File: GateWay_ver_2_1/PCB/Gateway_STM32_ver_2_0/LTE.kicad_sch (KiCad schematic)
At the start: 37 parts, among them J3 SIM_Card, Q2 MMBT3904, Q3 AO3400, Q4 AO3400, U6 SIM7600E-H

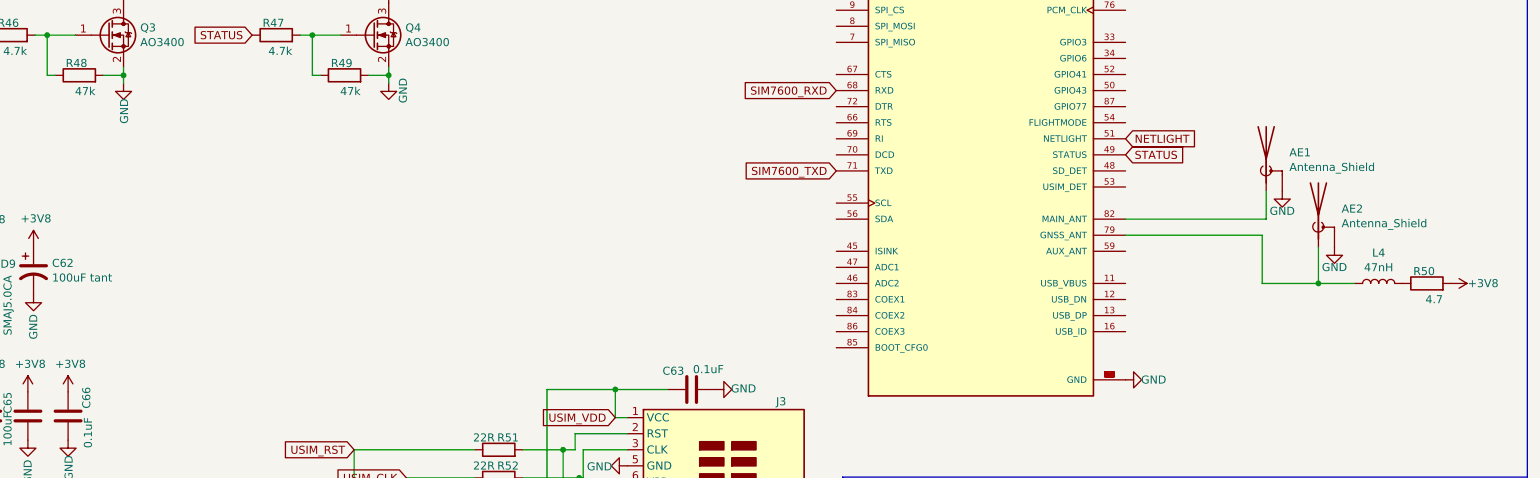
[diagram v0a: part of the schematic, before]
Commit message: 1
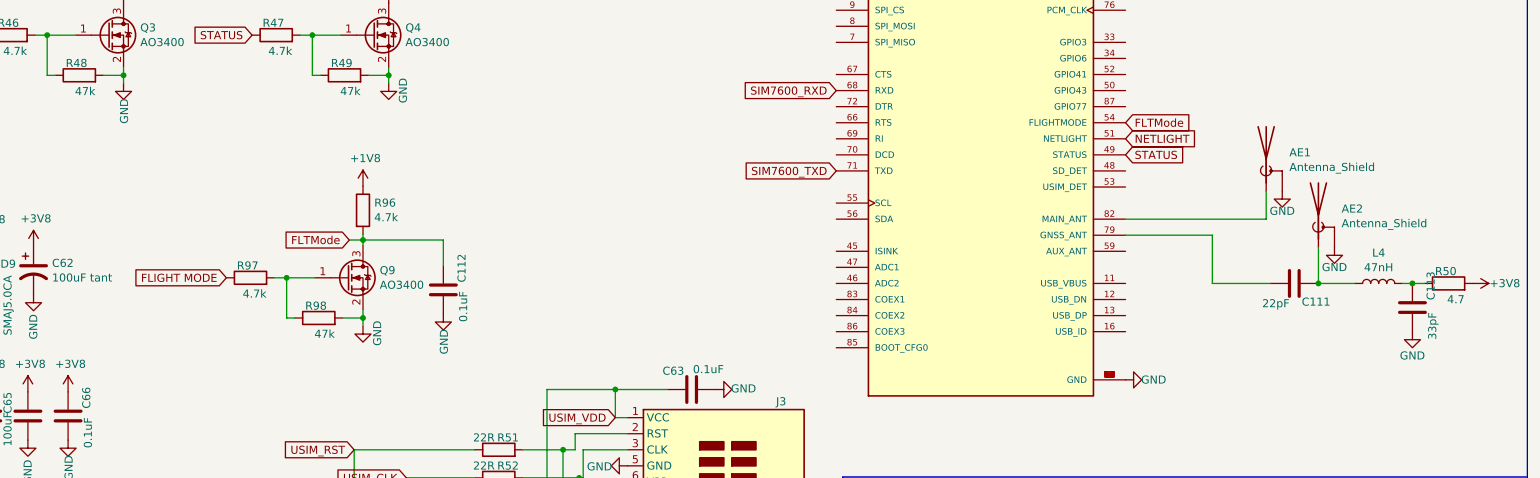
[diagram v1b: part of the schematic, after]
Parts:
- added C111: 22pF, Capacitor_SMD:C_0603_1608Metric, symbol Device:C
- added C112: 0.1uF, Capacitor_SMD:C_0603_1608Metric, symbol Device:C
- added C113: 33pF, Capacitor_SMD:C_0603_1608Metric, symbol Device:C
- added Q9: AO3400, Package_TO_SOT_SMD:SOT-23, symbol Transistor_FET:BSS138
- added R96, R97: 4.7k, Resistor_SMD:R_0603_1608Metric, symbol Device:R
- added R98: 47k, Resistor_SMD:R_0603_1608Metric, symbol Device:R
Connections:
- net +1V8: now also R96.1
- net GND: now also C112.2, C113.2, Q9.2 (S), R98.2
- net at AE2.1 (A), L4.1: now also C111.1; no longer U6.79 (GNSS_ANT)
- net at L4.2, R50.1: now also C113.1
- net FLTMode: now reaches U6.54 (FLIGHTMODE)
- net FLTMode: now also C112.1, Q9.3 (D), R96.2
- new net: Q9.1 (G), R97.2, R98.1
- new net: C111.2, U6.79 (GNSS_ANT)
- new net FLIGHT MODE: R97.1
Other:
- moved on the sheet: R50
